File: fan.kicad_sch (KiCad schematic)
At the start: 15 parts, among them J6 Conn_01x04, J7 Conn_01x04, U10 EMC2101

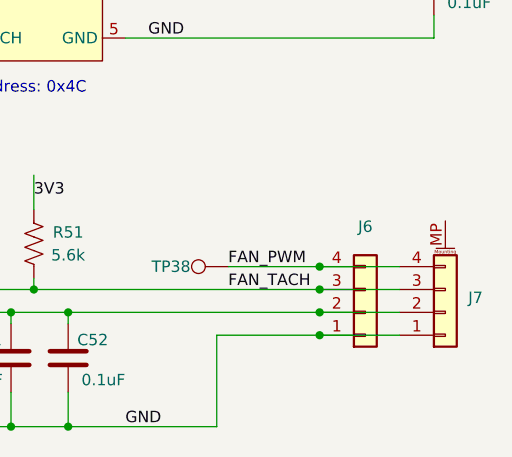
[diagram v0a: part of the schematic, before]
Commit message: layout
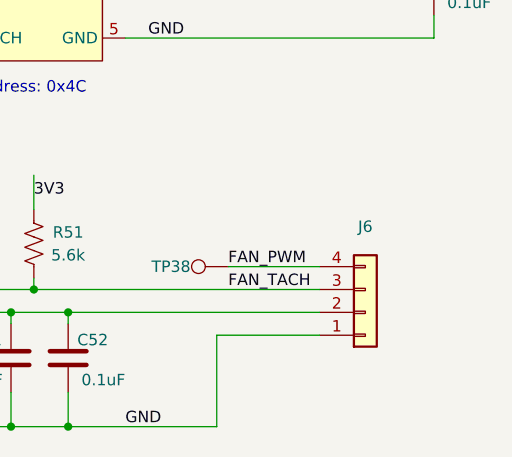
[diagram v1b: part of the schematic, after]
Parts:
- removed J7: Conn_01x04, Connector_JST:JST_SH_BM04B-SRSS-TB_1x04-1MP_P1.00mm_Vertical, symbol Connector_Generic_MountingPin:Conn_01x04_MountingPin
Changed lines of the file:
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@@
-	)
-	(junction
-		(at 179.07 114.3)
-		(diameter 0)
-		(color 0 0 0 0)
 	)
 	(junction
@@
 	)
 	(junction
-		(at 179.07 111.76)
-		(diameter 0)
-		(color 0 0 0 0)
-	)
-	(junction
 		(at 106.68 86.36)
 		(diameter 0)
@@
 	)
 	(junction
-		(at 179.07 109.22)
-		(diameter 0)
-		(color 0 0 0 0)
-	)
-	(junction
 		(at 144.78 114.3)
-		(diameter 0)
-		(color 0 0 0 0)
-	)
-	(junction
-		(at 179.07 116.84)
 		(diameter 0)
 		(color 0 0 0 0)
@@
 	(wire
 		(pts
-			(xy 179.07 111.76) (xy 187.96 111.76)
-		)
-		(stroke
-			(width 0)
-			(type default)
-		)
-	)
-	(wire
-		(pts
 			(xy 151.13 127) (xy 167.64 127)
 		)
@@
 	(wire
 		(pts
-			(xy 179.07 116.84) (xy 187.96 116.84)
-		)
-		(stroke
-			(width 0)
-			(type default)
-		)
-	)
-	(wire
-		(pts
 			(xy 179.07 66.04) (xy 191.77 66.04)
 		)
@@
 	(wire
 		(pts
-			(xy 179.07 114.3) (xy 187.96 114.3)
-		)
-		(stroke
-			(width 0)
-			(type default)
-		)
-	)
-	(wire
-		(pts
 			(xy 157.48 83.82) (xy 191.77 83.82)
 		)
@@
 		(pts
 			(xy 134.62 127) (xy 144.78 127)
-		)
-		(stroke
-			(width 0)
-			(type default)
-		)
-	)
-	(wire
-		(pts
-			(xy 179.07 109.22) (xy 187.96 109.22)
 		)
 		(stroke
@@
 					(unit 1)
 				)
-			)
-		)
-	)
-	(symbol
-		(lib_id "Connector_Generic_MountingPin:Conn_01x04_MountingPin")
-		(at 193.04 114.3 0)
-		(mirror x)
-		(unit 1)
-		(exclude_from_sim no)
-		(in_bom yes)
-		(on_board yes)
-		(dnp no)
-		(fields_autoplaced yes)
-		(property "Reference" "J7"
-			(at 195.58 112.6743 0)
-			(effects
-				(font
-					(size 1.27 1.27)
-				)
-				(justify left)
-			)
-		)
-		(property "Value" "Conn_01x04"
-			(at 193.04 104.775 0)
-			(effects
-				(font
-					(size 1.27 1.27)
-				)
-				(hide yes)
-			)
-		)
-		(property "Footprint" "Connector_JST:JST_SH_BM04B-SRSS-TB_1x04-1MP_P1.00mm_Vertical"
-			(at 193.04 114.3 0)
-			(effects
-				(font
-					(size 1.27 1.27)
-				)
-				(hide yes)
-			)
-		)
-		(property "Datasheet" "~"
-			(at 193.04 114.3 0)
-			(effects
-				(font
-					(size 1.27 1.27)
-				)
-				(hide yes)
-			)
-		)
-		(property "Description" "Generic connectable mounting pin connector, single row, 01x04, script generated (kicad-library-utils/schlib/autogen/connector/)"
-			(at 193.04 114.3 0)
-			(effects
-				(font
-					(size 1.27 1.27)
-				)
-				(hide yes)
-			)
-		)
-		(property "PARTNO" ""
-			(at 193.04 114.3 0)
-			(effects
-				(font
-					(size 1.27 1.27)
-				)
-				(hide yes)
-			)
-		)
-		(property "DK" ""
-			(at 193.04 114.3 0)
-			(effects
-				(font
-					(size 1.27 1.27)
-				)
-				(hide yes)
-			)
-		)
-		(pin "1"
-		)
-		(pin "2"
-		)
-		(pin "3"
-		)
-		(pin "4"
-		)
-		(pin "MP"
-		)
-		(instances
-			(project "bitaxeGamma"
-				(path "/e63e39d7-6ac0-4ffd-8aa3-1841a4541b55/8e8832ea-6bf1-49d2-b3a5-32a207f555d2"
-					(reference "J7")
-					(unit 1)
-				)

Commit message: DRC/layout
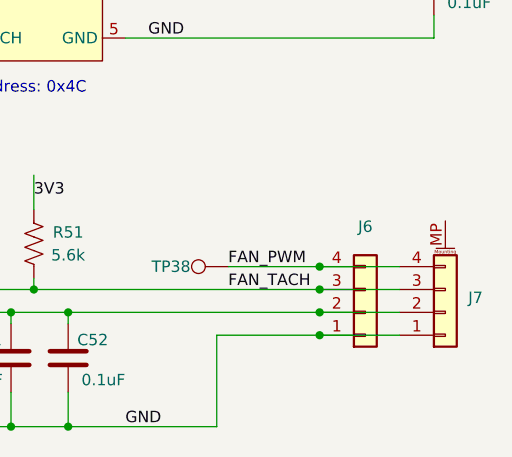
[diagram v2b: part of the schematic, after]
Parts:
- added J7: Conn_01x04, Connector_JST:JST_SH_BM04B-SRSS-TB_1x04-1MP_P1.00mm_Vertical, symbol Connector_Generic_MountingPin:Conn_01x04_MountingPin
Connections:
- net 5V: now also J7.2 (Pin_2)
- net FAN_PWM: now also J7.4 (Pin_4)
- net FAN_TACH: now also J7.3 (Pin_3)
- net GND: now also J7.1 (Pin_1)
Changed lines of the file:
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@@
+	)
+	(junction
+		(at 179.07 116.84)
+		(diameter 0)
+		(color 0 0 0 0)
 	)
 	(junction
@@
 	)
 	(junction
+		(at 179.07 111.76)
+		(diameter 0)
+		(color 0 0 0 0)
+	)
+	(junction
 		(at 82.55 76.2)
 		(diameter 0)
@@
 	)
 	(junction
+		(at 179.07 109.22)
+		(diameter 0)
+		(color 0 0 0 0)
+	)
+	(junction
+		(at 179.07 114.3)
+		(diameter 0)
+		(color 0 0 0 0)
+	)
+	(junction
 		(at 106.68 73.66)
 		(diameter 0)
@@
 	(wire
 		(pts
+			(xy 179.07 109.22) (xy 187.96 109.22)
+		)
+		(stroke
+			(width 0)
+			(type default)
+		)
+	)
+	(wire
+		(pts
 			(xy 179.07 66.04) (xy 191.77 66.04)
 		)
@@
 	(wire
 		(pts
+			(xy 179.07 114.3) (xy 187.96 114.3)
+		)
+		(stroke
+			(width 0)
+			(type default)
+		)
+	)
+	(wire
+		(pts
 			(xy 191.77 66.04) (xy 191.77 73.66)
 		)
@@
 	(wire
 		(pts
+			(xy 179.07 116.84) (xy 187.96 116.84)
+		)
+		(stroke
+			(width 0)
+			(type default)
+		)
+	)
+	(wire
+		(pts
 			(xy 179.07 66.04) (xy 179.07 68.58)
 		)
@@
 		(pts
 			(xy 151.13 123.19) (xy 151.13 127)
+		)
+		(stroke
+			(width 0)
+			(type default)
+		)
+	)
+	(wire
+		(pts
+			(xy 179.07 111.76) (xy 187.96 111.76)
 		)
 		(stroke
@@
 					(unit 1)
 				)
+			)
+		)
+	)
+	(symbol
+		(lib_id "Connector_Generic_MountingPin:Conn_01x04_MountingPin")
+		(at 193.04 114.3 0)
+		(mirror x)
+		(unit 1)
+		(exclude_from_sim no)
+		(in_bom yes)
+		(on_board yes)
+		(dnp no)
+		(fields_autoplaced yes)
+		(property "Reference" "J7"
+			(at 195.58 112.6743 0)
+			(effects
+				(font
+					(size 1.27 1.27)
+				)
+				(justify left)
+			)
+		)
+		(property "Value" "Conn_01x04"
+			(at 193.04 104.775 0)
+			(effects
+				(font
+					(size 1.27 1.27)
+				)
+				(hide yes)
+			)
+		)
+		(property "Footprint" "Connector_JST:JST_SH_BM04B-SRSS-TB_1x04-1MP_P1.00mm_Vertical"
+			(at 193.04 114.3 0)
+			(effects
+				(font
+					(size 1.27 1.27)
+				)
+				(hide yes)
+			)
+		)
+		(property "Datasheet" "~"
+			(at 193.04 114.3 0)
+			(effects
+				(font
+					(size 1.27 1.27)
+				)
+				(hide yes)
+			)
+		)
+		(property "Description" "Generic connectable mounting pin connector, single row, 01x04, script generated (kicad-library-utils/schlib/autogen/connector/)"
+			(at 193.04 114.3 0)
+			(effects
+				(font
+					(size 1.27 1.27)
+				)
+				(hide yes)
+			)
+		)
+		(property "PARTNO" ""
+			(at 193.04 114.3 0)
+			(effects
+				(font
+					(size 1.27 1.27)
+				)
+				(hide yes)
+			)
+		)
+		(property "DK" ""
+			(at 193.04 114.3 0)
+			(effects
+				(font
+					(size 1.27 1.27)
+				)
+				(hide yes)
+			)
+		)
+		(pin "1"
+		)
+		(pin "2"
+		)
+		(pin "3"
+		)
+		(pin "4"
+		)
+		(pin "MP"
+		)
+		(instances
+			(project "bitaxeGamma"
+				(path "/e63e39d7-6ac0-4ffd-8aa3-1841a4541b55/8e8832ea-6bf1-49d2-b3a5-32a207f555d2"
+					(reference "J7")
+					(unit 1)
+				)
